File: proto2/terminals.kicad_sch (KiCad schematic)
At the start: 118 parts, among them J1 Output 1, J10 Output, J11 Device, J12 Output, J2 Main Power, J3 Output, J4 Output, J5 Device, J6 Output, J7 Device, J8 Output, J9 Device

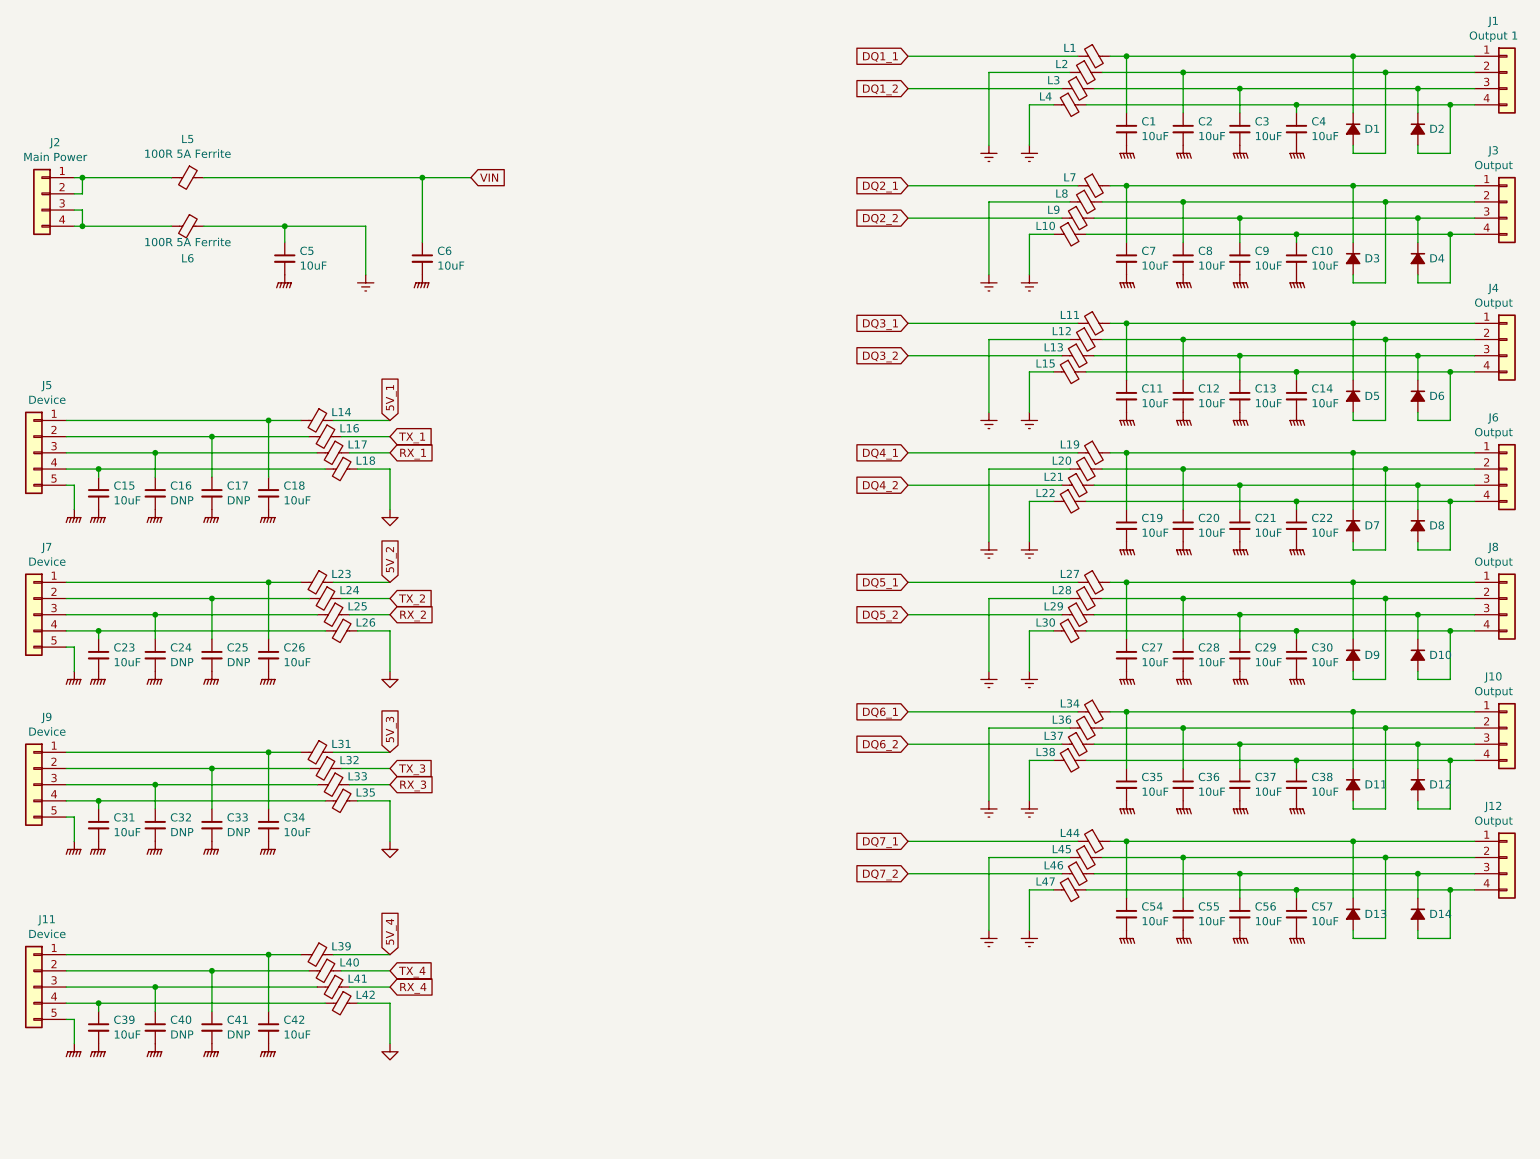
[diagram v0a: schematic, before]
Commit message: Working in suggestions from CFL review.
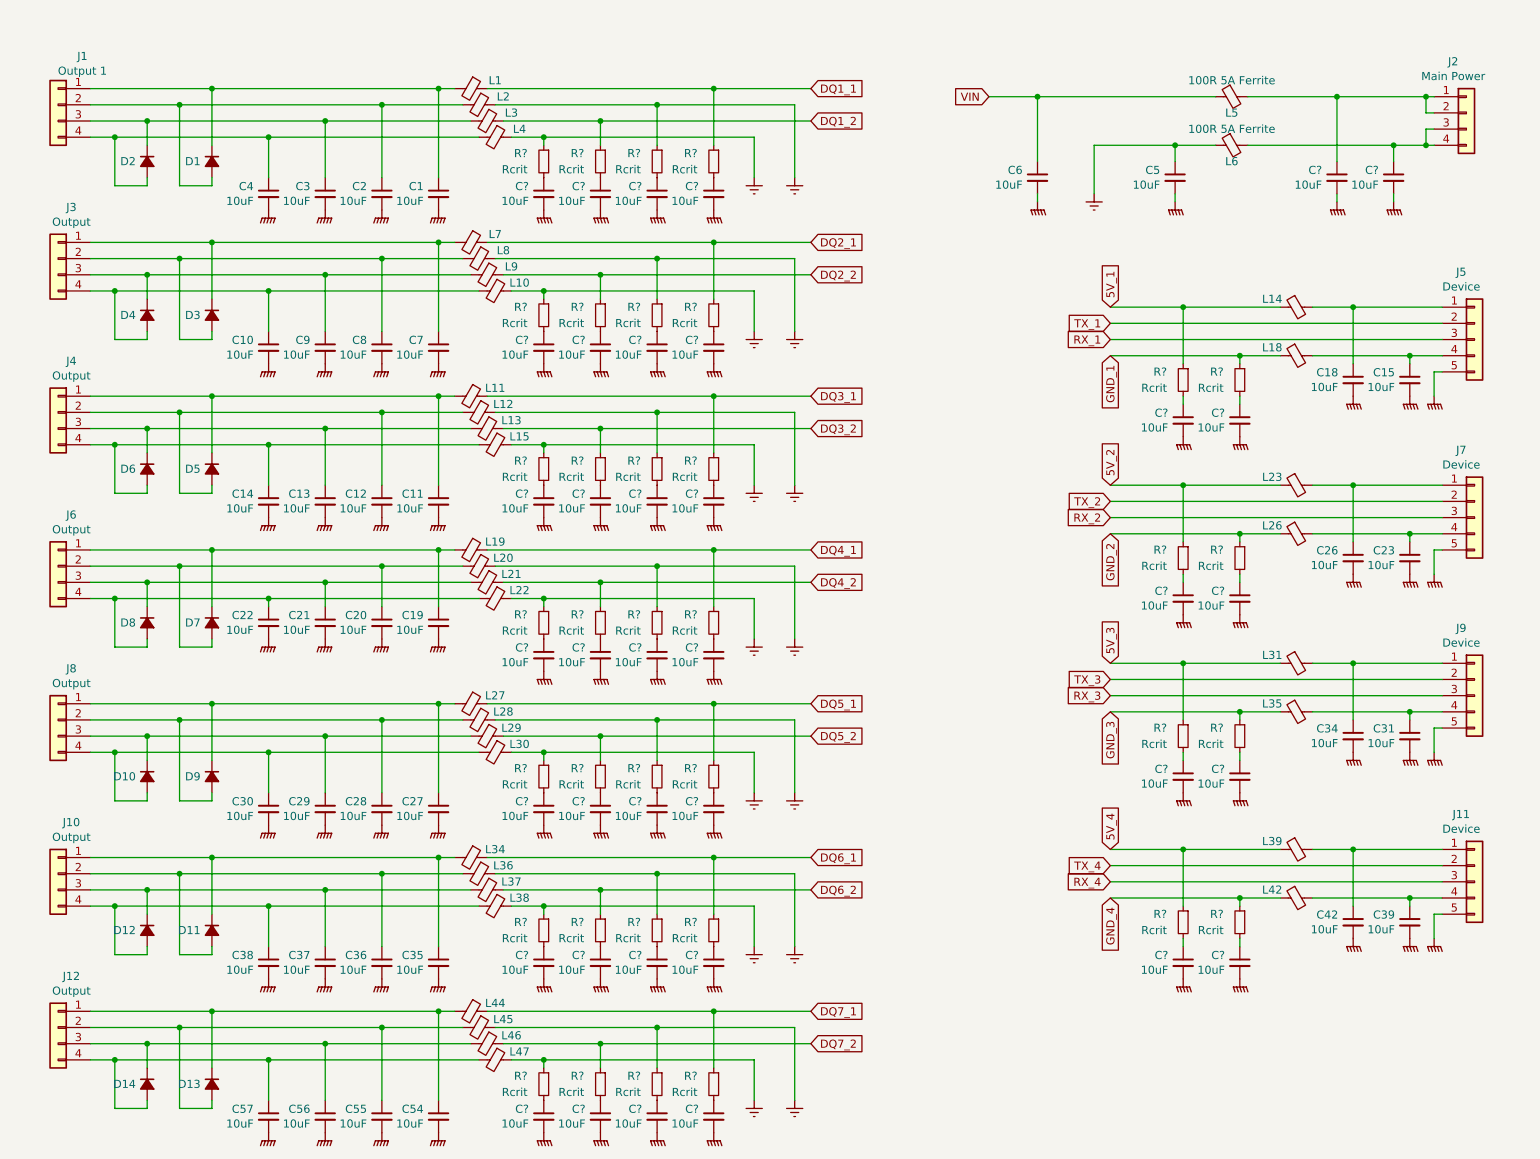
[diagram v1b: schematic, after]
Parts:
- removed C16, C17, C24, C25, C32, C33, C40, C41: DNP, Capacitor_SMD:C_0805_2012Metric, symbol Device:C_Small
- removed L16, L17, L24, L25, L32, L33, L40, L41: 0R, Resistor_SMD:R_0805_2012Metric, symbol Device:Ferrite_Bead_Small
- added C? (x38): 10uF, Capacitor_SMD:C_0805_2012Metric, symbol Device:C_Small
- added R? (x36): Rcrit, symbol Device:R_Small
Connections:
- net 5V_1: now also R?.1
- net 5V_2: now also R?.1
- net 5V_3: now also R?.1
- net 5V_4: now also R?.1
- net DQ1_1: now also R?.1
- net DQ1_2: now also R?.1
- net DQ2_1: now also R?.1
- net DQ2_2: now also R?.1
- net DQ3_1: now also R?.1
- net DQ3_2: now also R?.1
- net DQ4_1: now also R?.1
- net DQ4_2: now also R?.1
- net DQ5_1: now also R?.1
- net DQ5_2: now also R?.1
- net DQ6_1: now also R?.1
- net DQ6_2: now also R?.1
- net DQ7_1: now also R?.1
- net DQ7_2: now also R?.1
- net Earth: now also R?.1, R?.1, R?.1, R?.1, R?.1, R?.1, R?.1, R?.1, R?.1, R?.1, R?.1, R?.1, R?.1, R?.1
- net GNDPWR: now also C?.2, C?.2, C?.2, C?.2, C?.2, C?.2, C?.2, C?.2, C?.2, C?.2, C?.2, C?.2, C?.2, C?.2, C?.2, C?.2, C?.2, C?.2, C?.2, C?.2, C?.2, C?.2, C?.2, C?.2, C?.2, C?.2, C?.2, C?.2, C?.2, C?.2, C?.2, C?.2, C?.2, C?.2, C?.2, C?.2, C?.2, C?.2
- net RX_1: now also J5.3 (Pin_3)
- net RX_2: now also J7.3 (Pin_3)
- net RX_3: now also J9.3 (Pin_3)
- net RX_4: now also J11.3 (Pin_3)
- net TX_1: now also J5.2 (Pin_2)
- net TX_2: now also J7.2 (Pin_2)
- net TX_3: now also J9.2 (Pin_2)
- net TX_4: now also J11.2 (Pin_2)
- net at J2.1 (Pin_1), J2.2 (Pin_2), L5.2: now also C?.1
- net at J2.3 (Pin_3), J2.4 (Pin_4), L6.2: now also C?.1
- removed net GND: L18.1, L26.1, L35.1, L42.1
- new net: C?.1, R?.2 (x36)
- new net GND_1: L18.1, R?.1
- new net GND_2: L26.1, R?.1
- new net GND_3: L35.1, R?.1
- new net GND_4: L42.1, R?.1
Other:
- moved on the sheet: C1, C10, C11, C12, C13, C14, C15, C18, C19, C2, C20, C21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
